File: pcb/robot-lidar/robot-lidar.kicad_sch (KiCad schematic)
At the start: 29 parts, among them J2 YLIDAR X4, J3 Jack-DC, J5 Conn_02x03_Odd_Even, J7 Conn_ARM_SWD_TagConnect_TC2030, U1 STM32F429VETx, U2 LM317-3.3_SOT-223, U2 MPU-6050, Y1 Crystal

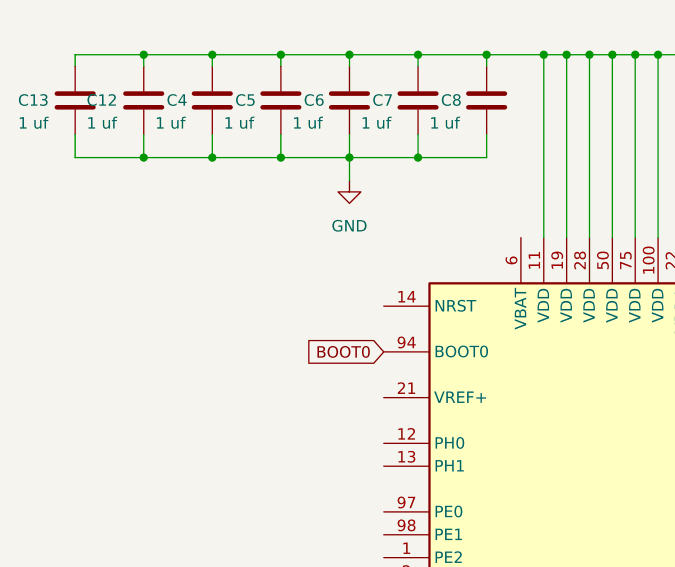
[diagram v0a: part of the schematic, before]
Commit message: add rst
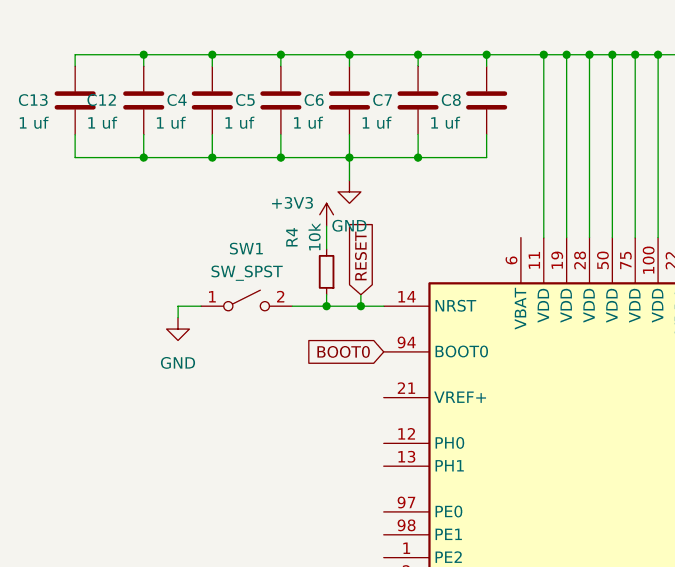
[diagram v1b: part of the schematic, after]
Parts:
- added R4: 10k, Resistor_SMD:R_0603_1608Metric, symbol Device:R_Small
- added SW1: SW_SPST, Button_Switch_SMD:SW_SPST_CK_RS282G05A3, symbol Switch:SW_SPST
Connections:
- net +3V3: now also R4.2
- net GND: now also SW1.1 (A)
- net RESET: now also U1.14 (NRST), R4.1, SW1.2 (B)
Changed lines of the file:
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@@
   (junction (at 237.49 97.79) (diameter 0) (color 0 0 0 0)
   )
+  (junction (at 52.07 49.53) (diameter 0) (color 0 0 0 0)
+  )
   (junction (at 85.09 21.59) (diameter 0) (color 0 0 0 0)
   )
@@
   (junction (at 242.57 59.69) (diameter 0) (color 0 0 0 0)
   )
+  (junction (at 48.26 49.53) (diameter 0) (color 0 0 0 0)
+  )
   (junction (at 236.22 -19.05) (diameter 0) (color 0 0 0 0)
   )
@@
     (stroke (width 0) (type default))
   )
+  (wire (pts (xy 52.07 49.53) (xy 54.61 49.53))
+    (stroke (width 0) (type default))
+  )
   (wire (pts (xy 87.63 21.59) (xy 87.63 41.91))
     (stroke (width 0) (type default))
   )
+  (wire (pts (xy 31.75 49.53) (xy 34.29 49.53))
+    (stroke (width 0) (type default))
+  )
   (wire (pts (xy 232.41 97.79) (xy 237.49 97.79))
     (stroke (width 0) (type default))
@@
     (stroke (width 0) (type default))
   )
+  (wire (pts (xy 48.26 49.53) (xy 52.07 49.53))
+    (stroke (width 0) (type default))
+  )
   (wire (pts (xy 229.87 -19.05) (xy 236.22 -19.05))
     (stroke (width 0) (type default))
@@
     (stroke (width 0) (type default))
   )
+  (wire (pts (xy 48.26 40.64) (xy 48.26 43.18))
+    (stroke (width 0) (type default))
+  )
   (wire (pts (xy 208.28 123.19) (xy 208.28 135.89))
     (stroke (width 0) (type default))
@@
     (stroke (width 0) (type default))
   )
+  (wire (pts (xy 48.26 49.53) (xy 48.26 48.26))
+    (stroke (width 0) (type default))
+  )
   (wire (pts (xy 261.62 59.69) (xy 270.51 59.69))
     (stroke (width 0) (type default))
@@
     (stroke (width 0) (type default))
   )
+  (wire (pts (xy 31.75 49.53) (xy 31.75 50.8))
+    (stroke (width 0) (type default))
+  )
   (wire (pts (xy 237.49 97.79) (xy 241.3 97.79))
     (stroke (width 0) (type default))
@@
     (stroke (width 0) (type default))
   )
+  (wire (pts (xy 44.45 49.53) (xy 48.26 49.53))
+    (stroke (width 0) (type default))
+  )
   (wire (pts (xy 77.47 184.15) (xy 77.47 190.5))
     (stroke (width 0) (type default))
@@
   )
   (wire (pts (xy 261.62 71.12) (xy 261.62 69.85))
+    (stroke (width 0) (type default))
+  )
+  (wire (pts (xy 52.07 48.26) (xy 52.07 49.53))
     (stroke (width 0) (type default))
   )
@@
     )
   )
+  (global_label "RESET" (shape input) (at 52.07 48.26 90) (fields_autoplaced)
+    (effects (font (size 1.27 1.27)) (justify left))
+    (property "Intersheetrefs" "${INTERSHEET_REFS}" (at 52.07 39.5297 90)
+      (effects (font (size 1.27 1.27)) (justify left) hide)
+    )
+  )
   (symbol (lib_id "Device:R_Small") (at 171.45 -16.51 270) (unit 1)
     (in_bom yes) (on_board yes) (dnp no)
@@
     )
   )
+  (symbol (lib_id "Switch:SW_SPST") (at 39.37 49.53 0) (unit 1)
+    (in_bom yes) (on_board yes) (dnp no) (fields_autoplaced)
+    (property "Reference" "SW1" (at 39.37 43.18 0)
+      (effects (font (size 1.27 1.27)))
+    )
+    (property "Value" "SW_SPST" (at 39.37 45.72 0)
+      (effects (font (size 1.27 1.27)))
+    )
+    (property "Footprint" "Button_Switch_SMD:SW_SPST_CK_RS282G05A3" (at 39.37 49.53 0)
+      (effects (font (size 1.27 1.27)) hide)
+    )
+    (property "Datasheet" "~" (at 39.37 49.53 0)
+      (effects (font (size 1.27 1.27)) hide)
+    )
+    (pin "1")
+    (pin "2")
+    (instances
+      (project "tablet"
+        (path "/868516f5-1ea3-47ae-b277-3f67998564bb"
+          (reference "SW1") (unit 1)
+        )
+      )
+      (project "robot-lidar"
+        (path "/cb10bbf7-c2c1-4a0d-8947-ad707931d83b"
+          (reference "SW1") (unit 1)
+        )
+      )
+    )
+  )
   (symbol (lib_id "Device:C") (at 270.51 128.27 0) (unit 1)
     (in_bom yes) (on_board yes) (dnp no) (fields_autoplaced)
@@
         (path "/cb10bbf7-c2c1-4a0d-8947-ad707931d83b"
           (reference "#PWR05") (unit 1)
+        )
+      )
+    )
+  )
+  (symbol (lib_id "Device:R_Small") (at 48.26 45.72 180) (unit 1)
+    (in_bom yes) (on_board yes) (dnp no)
+    (property "Reference" "R4" (at 44.45 41.91 90)
+      (effects (font (size 1.27 1.27)))
+    )
+    (property "Value" "10k" (at 46.99 41.91 90)
+      (effects (font (size 1.27 1.27)))
+    )
+    (property "Footprint" "Resistor_SMD:R_0603_1608Metric" (at 48.26 45.72 0)
+      (effects (font (size 1.27 1.27)) hide)
+    )
+    (property "Datasheet" "~" (at 48.26 45.72 0)
+      (effects (font (size 1.27 1.27)) hide)
+    )
+    (pin "1")
+    (pin "2")
+    (instances
+      (project "tablet"
+        (path "/868516f5-1ea3-47ae-b277-3f67998564bb"
+          (reference "R4") (unit 1)
+        )
+      )
+      (project "robot-lidar"
+        (path "/cb10bbf7-c2c1-4a0d-8947-ad707931d83b"
+          (reference "R7") (unit 1)
         )
       )
@@
     )
   )
+  (symbol (lib_id "power:+3V3") (at 48.26 40.64 0) (unit 1)
+    (in_bom yes) (on_board yes) (dnp no)
+    (property "Reference" "#PWR012" (at 48.26 44.45 0)
+      (effects (font (size 1.27 1.27)) hide)
+    )
+    (property "Value" "+3V3" (at 44.45 38.1 0)
+      (effects (font (size 1.27 1.27)))
+    )
+    (property "Footprint" "" (at 48.26 40.64 0)
+      (effects (font (size 1.27 1.27)) hide)
+    )
+    (property "Datasheet" "" (at 48.26 40.64 0)
+      (effects (font (size 1.27 1.27)) hide)
+    )
+    (pin "1")
+    (instances
+      (project "tablet"
+        (path "/868516f5-1ea3-47ae-b277-3f67998564bb"
+          (reference "#PWR012") (unit 1)
+        )
+      )
+      (project "robot-lidar"
+        (path "/cb10bbf7-c2c1-4a0d-8947-ad707931d83b"
+          (reference "#PWR021") (unit 1)
+        )
+      )
+    )
+  )
   (symbol (lib_id "power:+3V3") (at 115.57 -29.21 0) (unit 1)
     (in_bom yes) (on_board yes) (dnp no)
@@
         )
       )
+    )
+  )
+  (symbol (lib_id "power:GND") (at 31.75 50.8 0) (unit 1)
+    (in_bom yes) (on_board yes) (dnp no) (fields_autoplaced)
+    (property "Reference" "#PWR013" (at 31.75 57.15 0)
+      (effects (font (size 1.27 1.27)) hide)
+    )
+    (property "Value" "GND" (at 31.75 55.88 0)
+      (effects (font (size 1.27 1.27)))
+    )
+    (property "Footprint" "" (at 31.75 50.8 0)
+      (effects (font (size 1.27 1.27)) hide)
+    )
+    (property "Datasheet" "" (at 31.75 50.8 0)
+      (effects (font (size 1.27 1.27)) hide)
+    )
+    (pin "1")
+    (instances
+      (project "tablet"
+        (path "/868516f5-1ea3-47ae-b277-3f67998564bb"
+          (reference "#PWR013") (unit 1)
+        )
+      )
+      (project "robot-lidar"
+        (path "/cb10bbf7-c2c1-4a0d-8947-ad707931d83b"
+          (reference "#PWR020") (unit 1)
+        )
+      )
